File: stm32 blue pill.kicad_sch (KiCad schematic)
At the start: 23 parts

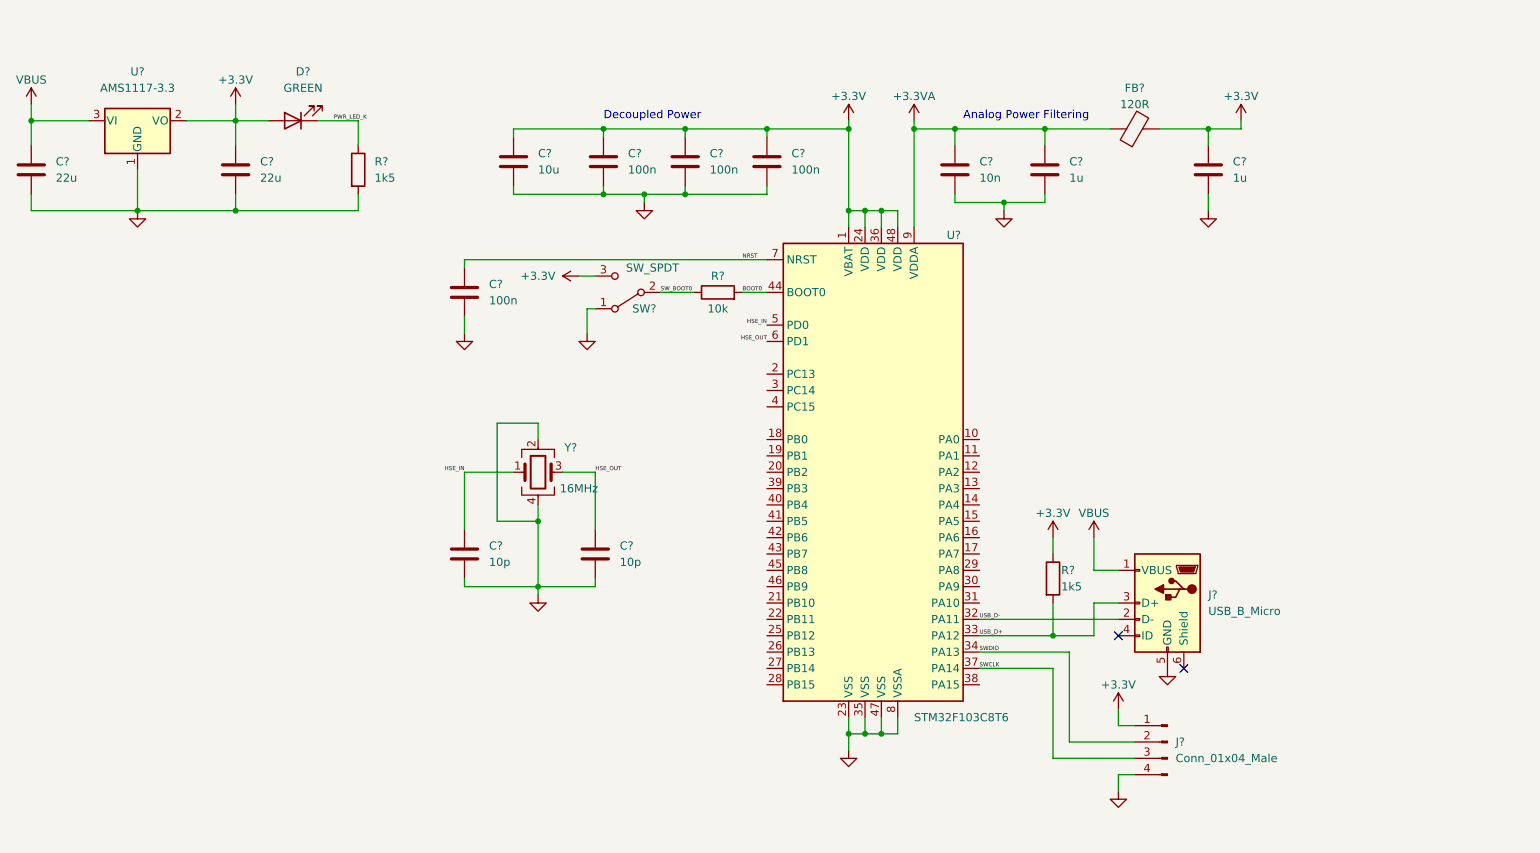
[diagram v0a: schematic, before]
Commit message: schematic updates & pcb init
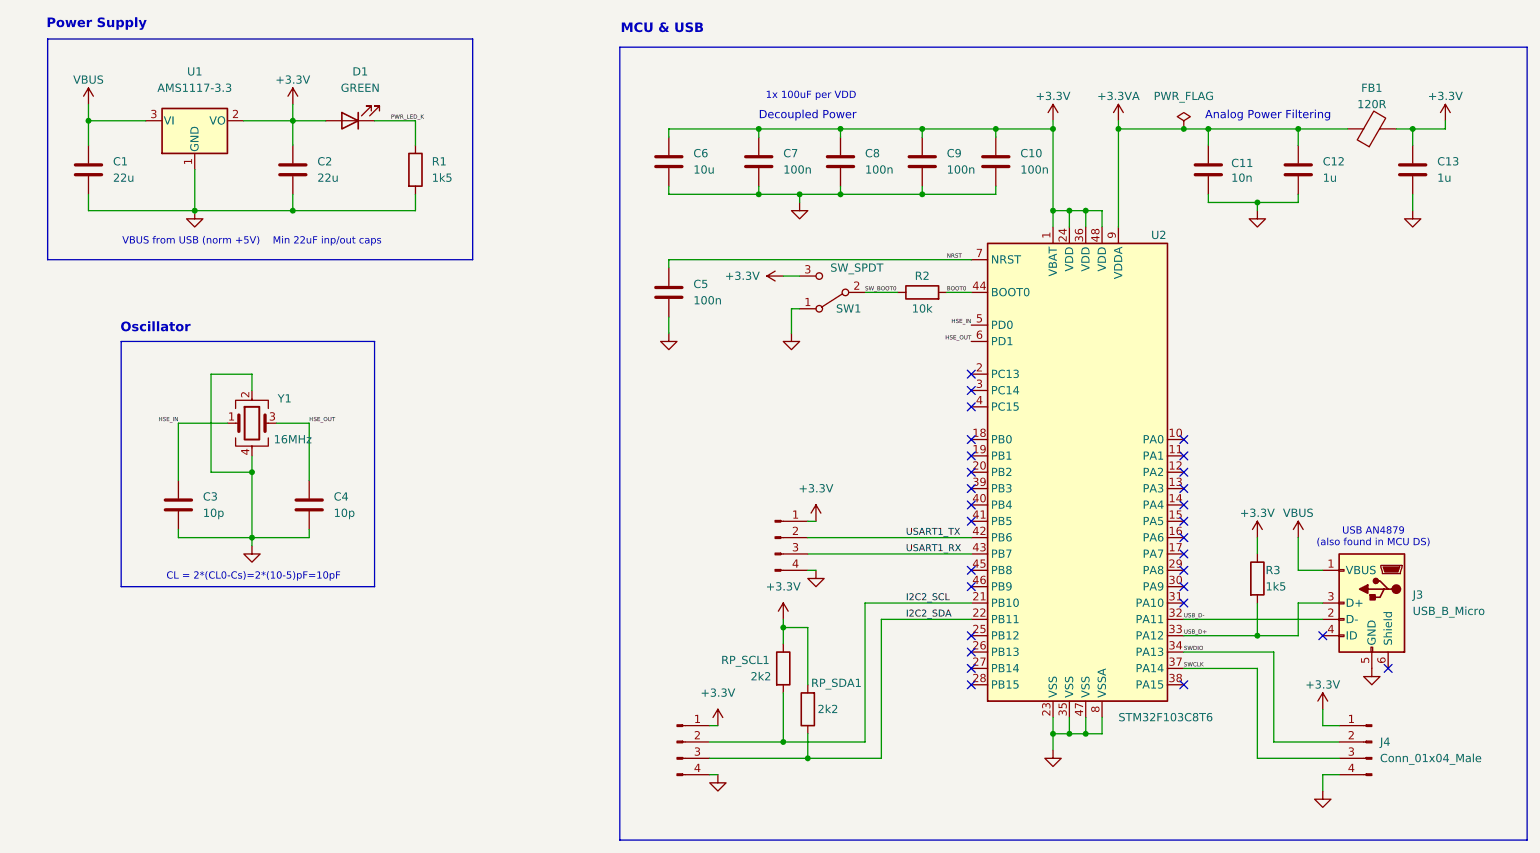
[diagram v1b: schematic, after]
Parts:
- added C10: 100n, Capacitor_SMD:C_0402_1005Metric, symbol Device:C
- added J1, J2: Conn_01x04_Male, Connector_PinHeader_2.00mm:PinHeader_1x04_P2.00mm_Vertical, symbol Connector:Conn_01x04_Male
- added RP_SCL1, RP_SDA1: 2k2, Resistor_SMD:R_0402_1005Metric, symbol Device:R
- C1, C2: renamed from C?; footprint (none) -> Capacitor_SMD:C_0805_2012Metric
- C11, C12, C13, C3, C4, C5, C7, C8, C9: renamed from C?; footprint (none) -> Capacitor_SMD:C_0402_1005Metric
- C6: renamed from C?; footprint (none) -> Capacitor_SMD:C_0603_1608Metric
- D1: renamed from D?; footprint (none) -> LED_SMD:LED_0603_1608Metric
- FB1: renamed from FB?; footprint (none) -> Inductor_SMD:L_0603_1608Metric
- J3: renamed from J?; footprint (none) -> Connector_USB:USB_Micro-B_Wuerth_629105150521
- J4: renamed from J?; footprint (none) -> Connector_PinHeader_2.00mm:PinHeader_1x04_P2.00mm_Vertical
- R1, R2, R3: renamed from R?; footprint (none) -> Resistor_SMD:R_0402_1005Metric
- SW1: renamed from SW?; footprint (none) -> Button_Switch_SMD:SW_SPDT_PCM12
- Y1: renamed from Y?; footprint (none) -> Crystal:Crystal_SMD_3225-4Pin_3.2x2.5mm
- gave numbers to parts that had none: 2
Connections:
- net +3.3V: now also C10.1, J1.1 (Pin_1), J2.1 (Pin_1), RP_SCL1.1, RP_SDA1.2
- net GND: now also C10.2, J1.4 (Pin_4), J2.4 (Pin_4)
- net I2C2_SCL: now reaches U2.21 (PB10)
- net I2C2_SCL: now also J2.2 (Pin_2), RP_SCL1.2
- net I2C2_SDA: now reaches U2.22 (PB11)
- net I2C2_SDA: now also J2.3 (Pin_3), RP_SDA1.1
- net USART1_TX: now reaches U2.42 (PB6)
- net USART1_TX: now also J1.2 (Pin_2)
- net USART1_RX: now reaches U2.43 (PB7)
- net USART1_RX: now also J1.3 (Pin_3)
- no-connect marks 2 -> 29
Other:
- note added: "1x 100uF per VDD"
- note added: "CL = 2*(CL0-Cs)=2*(10-5)pF=10pF"
- note added: "MCU & USB"
- note added: "Oscillator"
- note added: "Power Supply"
- note added: "USB AN4879 (also found in MCU DS)"
- note added: "VBUS from USB (norm +5V) Min 22uF inp/out caps"
- title: (none) -> Blue Pill (Minimal)
- moved on the sheet: C1, C11, C12, C13, C2, C3, C4, C5, C6, C7, C8, C9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
